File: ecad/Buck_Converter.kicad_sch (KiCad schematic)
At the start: 10 parts, among them SW1 SW_SPST, U1 MCP16331x-xCH

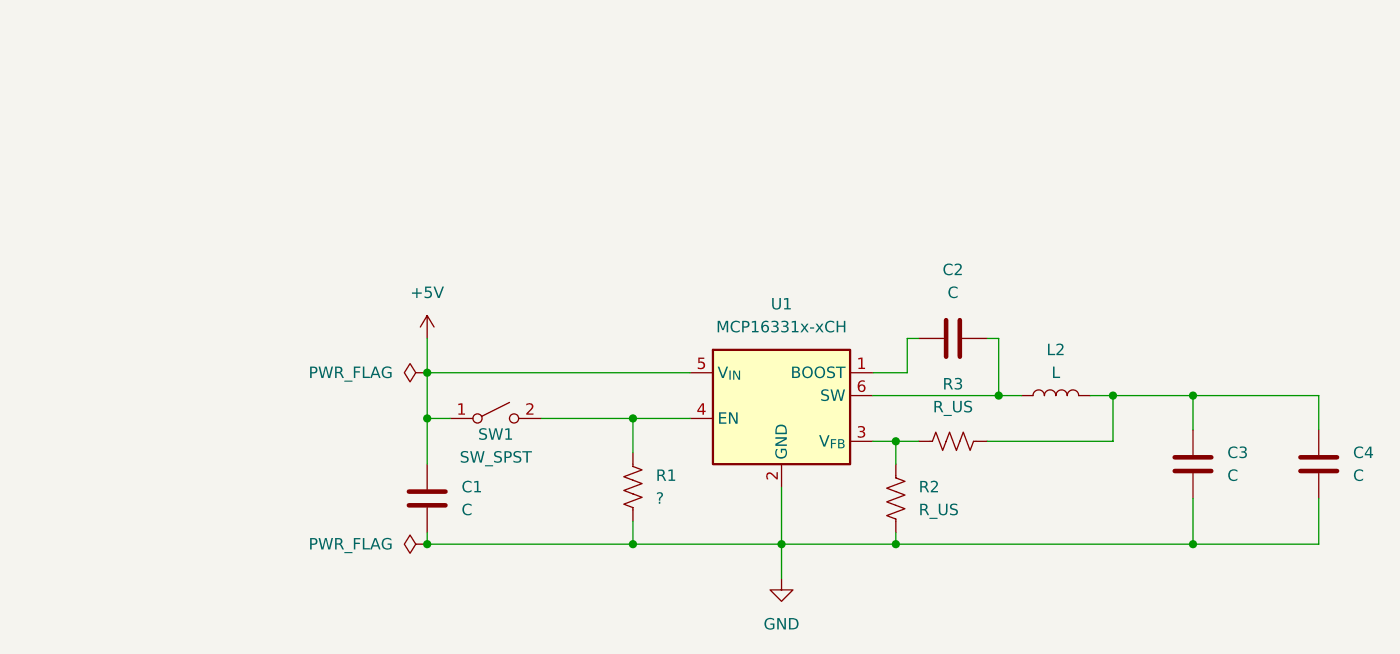
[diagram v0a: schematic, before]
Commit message: To add front panel
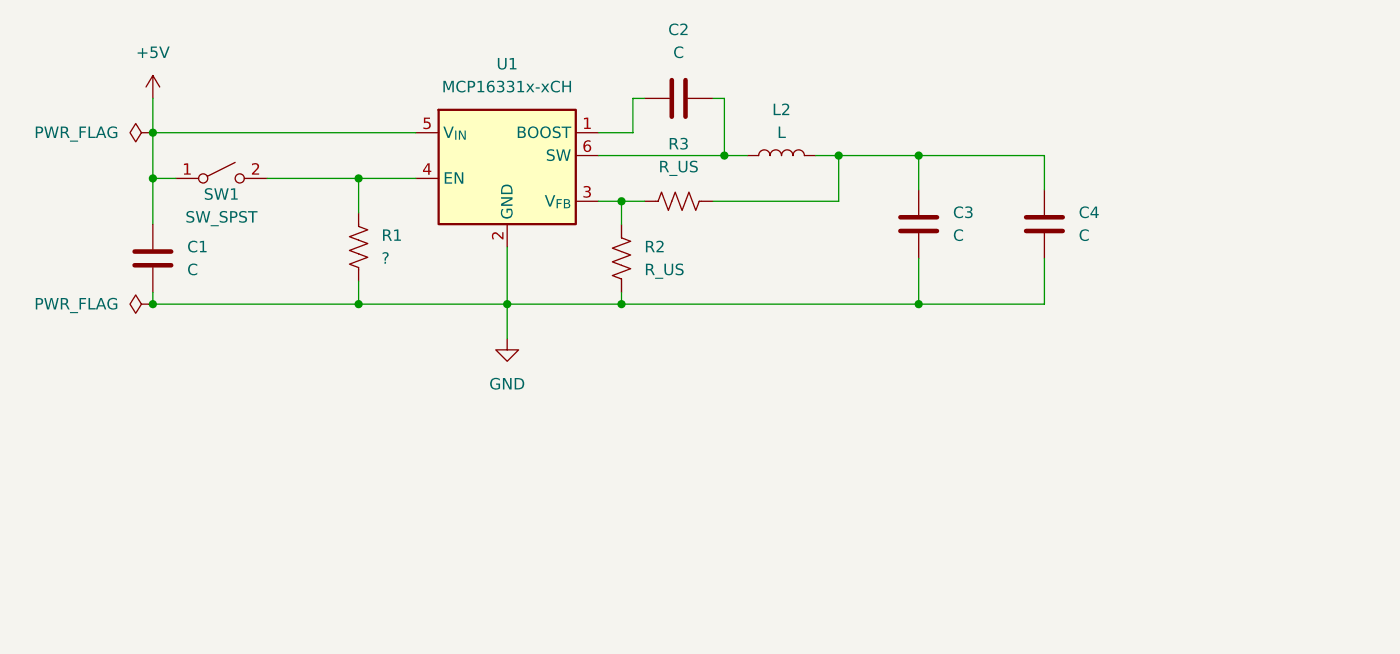
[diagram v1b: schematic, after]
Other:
- title: (none) -> Buck Converter
- moved on the sheet: C1, C2, C3, C4, L2, R1, R2, R3, SW1, U1
